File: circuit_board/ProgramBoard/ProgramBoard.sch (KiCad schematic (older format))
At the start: 7 parts, among them J1 BARREL_JACK, P1 IDC-10, P2 HEADER_6, P3 HEADER_3, P4 HEADER_3, P5 HEADER_3, U1 SparkFun_FT231X_Breakout

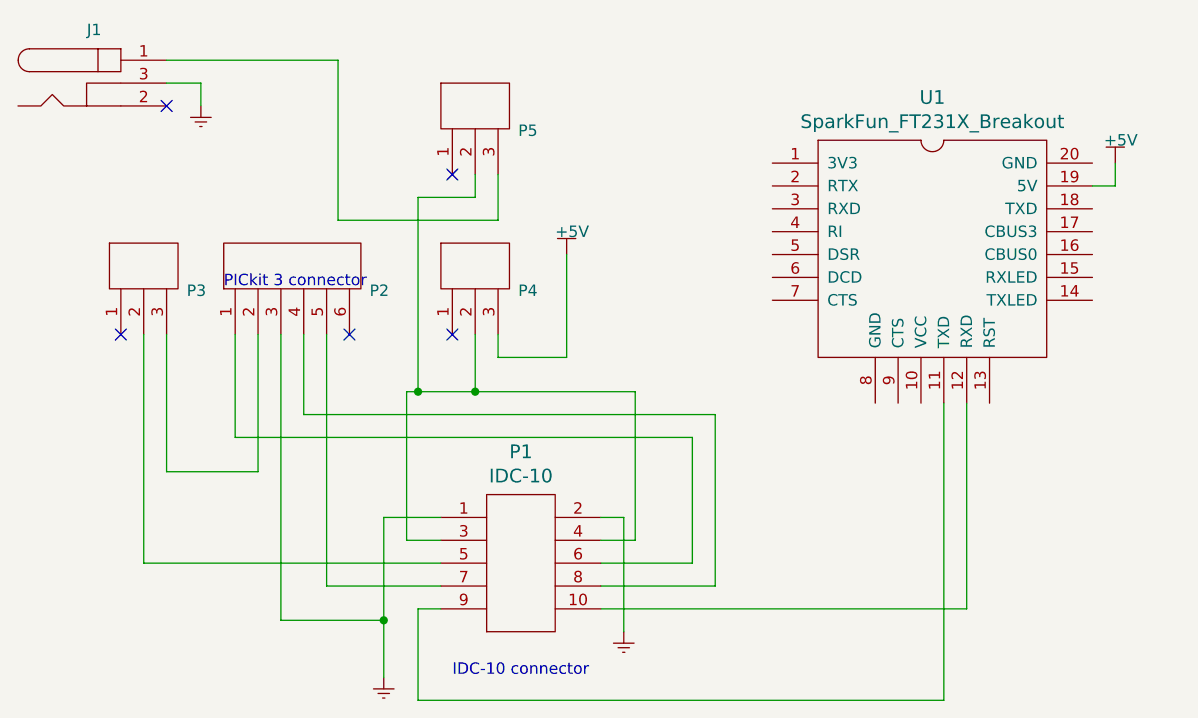
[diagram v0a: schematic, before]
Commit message: Revert "Revert "Merge branch 'master' of https://github.com/zrs5532/mri_demo""
This reverts commit c7bcd66b67d9c03c78e75f611b5453059c538dec.
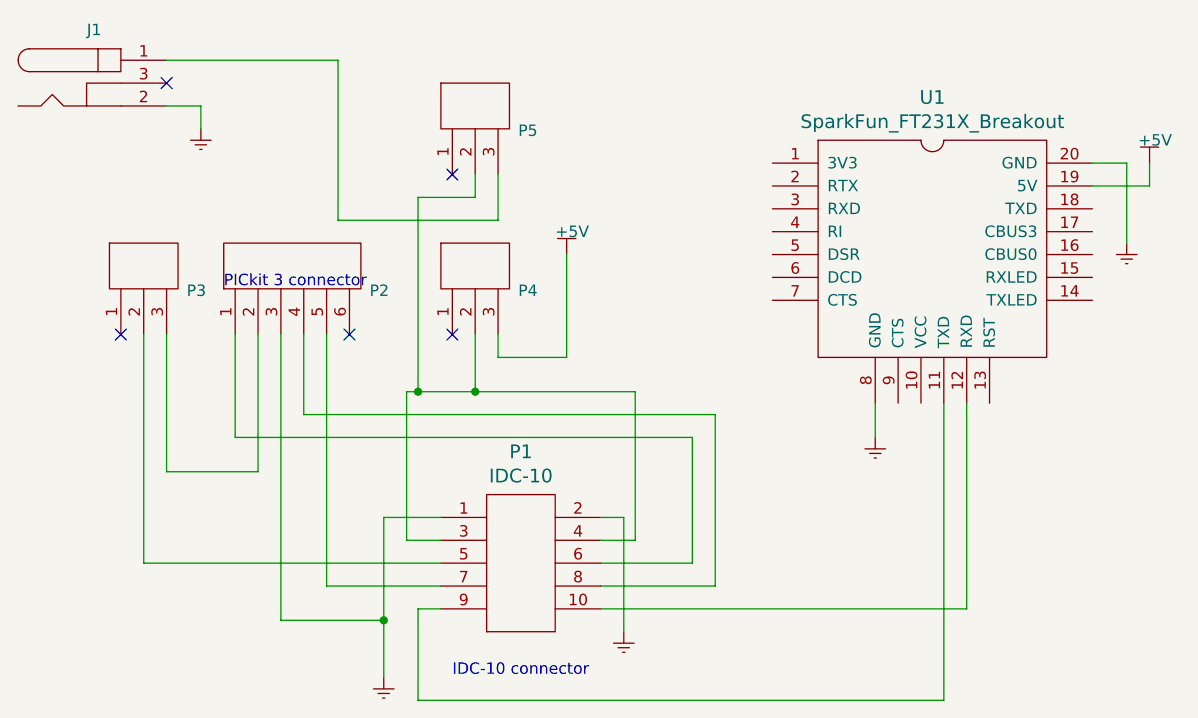
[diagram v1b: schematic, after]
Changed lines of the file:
@@
 L SensorDemo_power_supply:+5V #PS01
 U 1 1 603D79A0
-P 7600 3100
-F 0 "#PS01" H 7600 3050 50  0001 C CNN
-F 1 "+5V" H 7550 3200 50  0000 L CNN
-F 2 "" H 7605 2795 50  0001 C CNN
-F 3 "" H 7605 2795 50  0001 C CNN
-	1    7600 3100
-	1    0    0    -1
-$EndComp
-Wire Wire Line
-	7600 3100 7600 3200
-Wire Wire Line
-	7600 3200 7500 3200
+P 7750 3100
+F 0 "#PS01" H 7750 3050 50  0001 C CNN
+F 1 "+5V" H 7700 3200 50  0000 L CNN
+F 2 "" H 7755 2795 50  0001 C CNN
+F 3 "" H 7755 2795 50  0001 C CNN
+	1    7750 3100
+	1    0    0    -1
+$EndComp
+Wire Wire Line
+	7750 3100 7750 3200
+Wire Wire Line
+	7750 3200 7500 3200
 Wire Wire Line
 	5350 4650 5450 4650
@@
 	4650 4850 3350 4850
 $Comp
+L SensorDemo_connector:HEADER_3 P5
+U 1 1 6047EE8D
+P 4800 2850
+F 0 "P5" H 4988 2742 50  0000 L CNN
+F 1 "HEADER_3" H 4800 2300 50  0001 C CNN
+F 2 "SensorDemo_pcb:HEADER_3" H 8100 650 60  0001 C CNN
+F 3 "" H 8100 650 60  0000 C CNN
+	1    4800 2850
+	1    0    0    -1
+$EndComp
+NoConn ~ 4700 3150
+Wire Wire Line
+	4800 3150 4800 3250
+Wire Wire Line
+	4800 3250 4550 3250
+Wire Wire Line
+	4550 3250 4550 4100
+Connection ~ 4550 4100
+Wire Wire Line
+	4550 4100 4500 4100
+Wire Wire Line
+	4900 3150 4900 3350
+Wire Wire Line
+	4900 3350 4200 3350
+Wire Wire Line
+	4200 3350 4200 2650
+$Comp
+L SensorDemo_power_supply:GND #PS0102
+U 1 1 6049968C
+P 6550 4350
+F 0 "#PS0102" H 6550 4225 50  0001 C CNN
+F 1 "GND" H 6550 4275 50  0001 C CNN
+F 2 "" H 6550 4350 50  0001 C CNN
+F 3 "" H 6550 4350 50  0001 C CNN
+	1    6550 4350
+	1    0    0    -1
+$EndComp
+Wire Wire Line
+	6550 4150 6550 4300
+$Comp
+L SensorDemo_power_supply:GND #PS0103
+U 1 1 604A6DE7
+P 7650 3500
+F 0 "#PS0103" H 7650 3375 50  0001 C CNN
+F 1 "GND" H 7650 3425 50  0001 C CNN
+F 2 "" H 7650 3500 50  0001 C CNN
+F 3 "" H 7650 3500 50  0001 C CNN
+	1    7650 3500
+	1    0    0    -1
+$EndComp
+Wire Wire Line
+	7650 3100 7650 3450
+Wire Wire Line
+	7650 3100 7500 3100
+NoConn ~ 3450 2750
+Wire Wire Line
+	3600 2850 3450 2850
+Wire Wire Line
+	3600 2950 3600 2850
+$Comp
+L SensorDemo_power_supply:GND #PS0101
+U 1 1 6048CCC2
+P 3600 3000
+F 0 "#PS0101" H 3600 2875 50  0001 C CNN
+F 1 "GND" H 3600 2925 50  0001 C CNN
+F 2 "" H 3600 3000 50  0001 C CNN
+F 3 "" H 3600 3000 50  0001 C CNN
+	1    3600 3000
+	1    0    0    -1
+$EndComp
+Wire Wire Line
+	3450 2650 4200 2650
+$Comp
 L SensorDemo_connector:BARREL_JACK J1
 U 1 1 6047A3B5
@@
 	1    0    0    -1
 $EndComp
-$Comp
-L SensorDemo_connector:HEADER_3 P5
-U 1 1 6047EE8D
-P 4800 2850
-F 0 "P5" H 4988 2742 50  0000 L CNN
-F 1 "HEADER_3" H 4800 2300 50  0001 C CNN
-F 2 "SensorDemo_pcb:HEADER_3" H 8100 650 60  0001 C CNN
-F 3 "" H 8100 650 60  0000 C CNN
-	1    4800 2850
-	1    0    0    -1
-$EndComp
-NoConn ~ 4700 3150
-Wire Wire Line
-	4800 3150 4800 3250
-Wire Wire Line
-	4800 3250 4550 3250
-Wire Wire Line
-	4550 3250 4550 4100
-Connection ~ 4550 4100
-Wire Wire Line
-	4550 4100 4500 4100
-Wire Wire Line
-	4900 3150 4900 3350
-Wire Wire Line
-	4900 3350 4200 3350
-Wire Wire Line
-	4200 3350 4200 2650
-Wire Wire Line
-	3450 2650 4200 2650
-$Comp
-L SensorDemo_power_supply:GND #PS?
-U 1 1 6048CCC2
-P 3600 2900
-F 0 "#PS?" H 3600 2775 50  0001 C CNN
-F 1 "GND" H 3600 2825 50  0001 C CNN
-F 2 "" H 3600 2900 50  0001 C CNN
-F 3 "" H 3600 2900 50  0001 C CNN
-	1    3600 2900
-	1    0    0    -1
-$EndComp
-Wire Wire Line
-	3600 2850 3600 2750
-Wire Wire Line
-	3600 2750 3450 2750
-NoConn ~ 3450 2850
 $EndSCHEMATC

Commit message: Revert "Merge branch 'master' of https://github.com/zrs5532/mri_demo"
This reverts commit b0c8028f714b16f114d60085c0a86ac2043fc740, reversing
changes made to 0fccd9f34ae5c363ed48057d6b873a7540cc24aa.
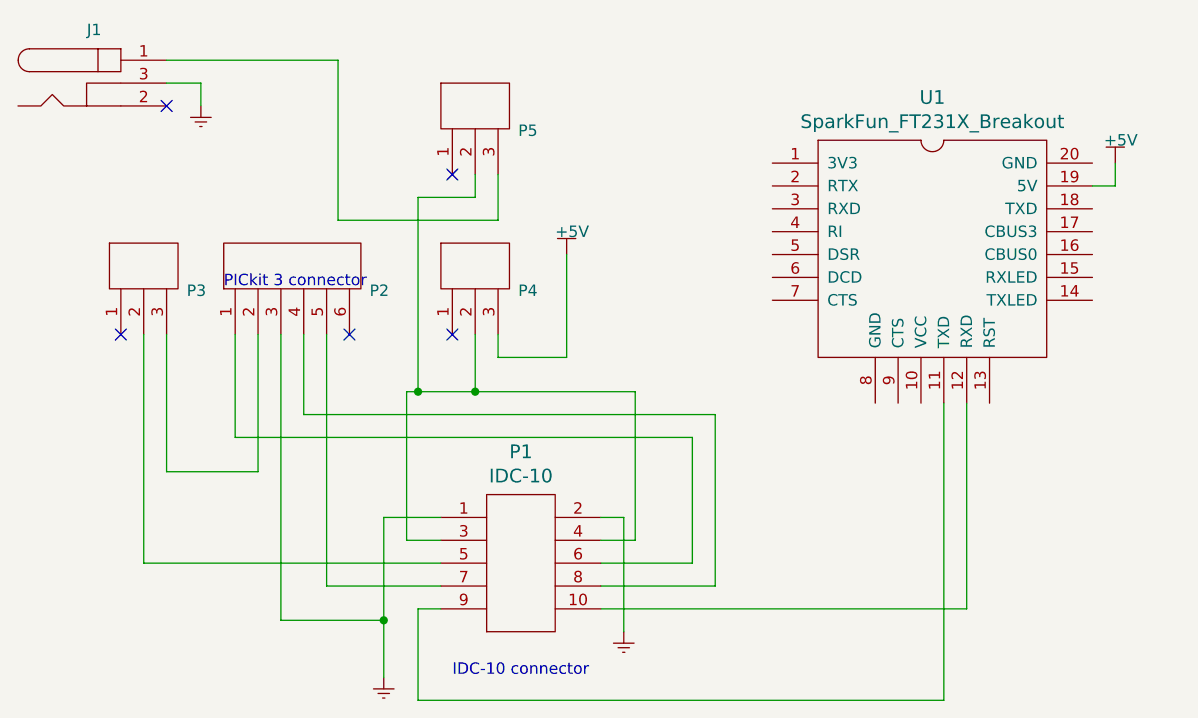
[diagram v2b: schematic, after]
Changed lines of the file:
@@
 L SensorDemo_power_supply:+5V #PS01
 U 1 1 603D79A0
-P 7750 3100
-F 0 "#PS01" H 7750 3050 50  0001 C CNN
-F 1 "+5V" H 7700 3200 50  0000 L CNN
-F 2 "" H 7755 2795 50  0001 C CNN
-F 3 "" H 7755 2795 50  0001 C CNN
-	1    7750 3100
+P 7600 3100
+F 0 "#PS01" H 7600 3050 50  0001 C CNN
+F 1 "+5V" H 7550 3200 50  0000 L CNN
+F 2 "" H 7605 2795 50  0001 C CNN
+F 3 "" H 7605 2795 50  0001 C CNN
+	1    7600 3100
 	1    0    0    -1
 $EndComp
 Wire Wire Line
-	7750 3100 7750 3200
+	7600 3100 7600 3200
 Wire Wire Line
-	7750 3200 7500 3200
+	7600 3200 7500 3200
 Wire Wire Line
 	5350 4650 5450 4650
@@
 	4650 4850 3350 4850
 $Comp
+L SensorDemo_connector:BARREL_JACK J1
+U 1 1 6047A3B5
+P 3150 2750
+F 0 "J1" H 3133 2983 50  0000 C CNN
+F 1 "BARREL_JACK" H 3150 2550 50  0001 C CNN
+F 2 "SensorDemo_pcb:BARREL_JACK" H 3150 2750 60  0001 C CNN
+F 3 "" H 3150 2750 60  0000 C CNN
+	1    3150 2750
+	1    0    0    -1
+$EndComp
+$Comp
 L SensorDemo_connector:HEADER_3 P5
 U 1 1 6047EE8D
@@
 Wire Wire Line
 	4200 3350 4200 2650
+Wire Wire Line
+	3450 2650 4200 2650
 $Comp
-L SensorDemo_power_supply:GND #PS0102
-U 1 1 6049968C
-P 6550 4350
-F 0 "#PS0102" H 6550 4225 50  0001 C CNN
-F 1 "GND" H 6550 4275 50  0001 C CNN
-F 2 "" H 6550 4350 50  0001 C CNN
-F 3 "" H 6550 4350 50  0001 C CNN
-	1    6550 4350
+L SensorDemo_power_supply:GND #PS?
+U 1 1 6048CCC2
+P 3600 2900
+F 0 "#PS?" H 3600 2775 50  0001 C CNN
+F 1 "GND" H 3600 2825 50  0001 C CNN
+F 2 "" H 3600 2900 50  0001 C CNN
+F 3 "" H 3600 2900 50  0001 C CNN
+	1    3600 2900
 	1    0    0    -1
 $EndComp
 Wire Wire Line
-	6550 4150 6550 4300
-$Comp
-L SensorDemo_power_supply:GND #PS0103
-U 1 1 604A6DE7
-P 7650 3500
-F 0 "#PS0103" H 7650 3375 50  0001 C CNN
-F 1 "GND" H 7650 3425 50  0001 C CNN
-F 2 "" H 7650 3500 50  0001 C CNN
-F 3 "" H 7650 3500 50  0001 C CNN
-	1    7650 3500
-	1    0    0    -1
-$EndComp
+	3600 2850 3600 2750
 Wire Wire Line
-	7650 3100 7650 3450
-Wire Wire Line
-	7650 3100 7500 3100
-NoConn ~ 3450 2750
-Wire Wire Line
-	3600 2850 3450 2850
-Wire Wire Line
-	3600 2950 3600 2850
-$Comp
-L SensorDemo_power_supply:GND #PS0101
-U 1 1 6048CCC2
-P 3600 3000
-F 0 "#PS0101" H 3600 2875 50  0001 C CNN
-F 1 "GND" H 3600 2925 50  0001 C CNN
-F 2 "" H 3600 3000 50  0001 C CNN
-F 3 "" H 3600 3000 50  0001 C CNN
-	1    3600 3000
-	1    0    0    -1
-$EndComp
-Wire Wire Line
-	3450 2650 4200 2650
-$Comp
-L SensorDemo_connector:BARREL_JACK J1
-U 1 1 6047A3B5
-P 3150 2750
-F 0 "J1" H 3133 2983 50  0000 C CNN
-F 1 "BARREL_JACK" H 3150 2550 50  0001 C CNN
-F 2 "SensorDemo_pcb:BARREL_JACK" H 3150 2750 60  0001 C CNN
-F 3 "" H 3150 2750 60  0000 C CNN
-	1    3150 2750
-	1    0    0    -1
-$EndComp
+	3600 2750 3450 2750
+NoConn ~ 3450 2850
 $EndSCHEMATC
